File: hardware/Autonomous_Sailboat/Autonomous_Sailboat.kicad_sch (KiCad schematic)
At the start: 16 parts, among them Q1 Q_NMOS, U1 STM32H755ZITx

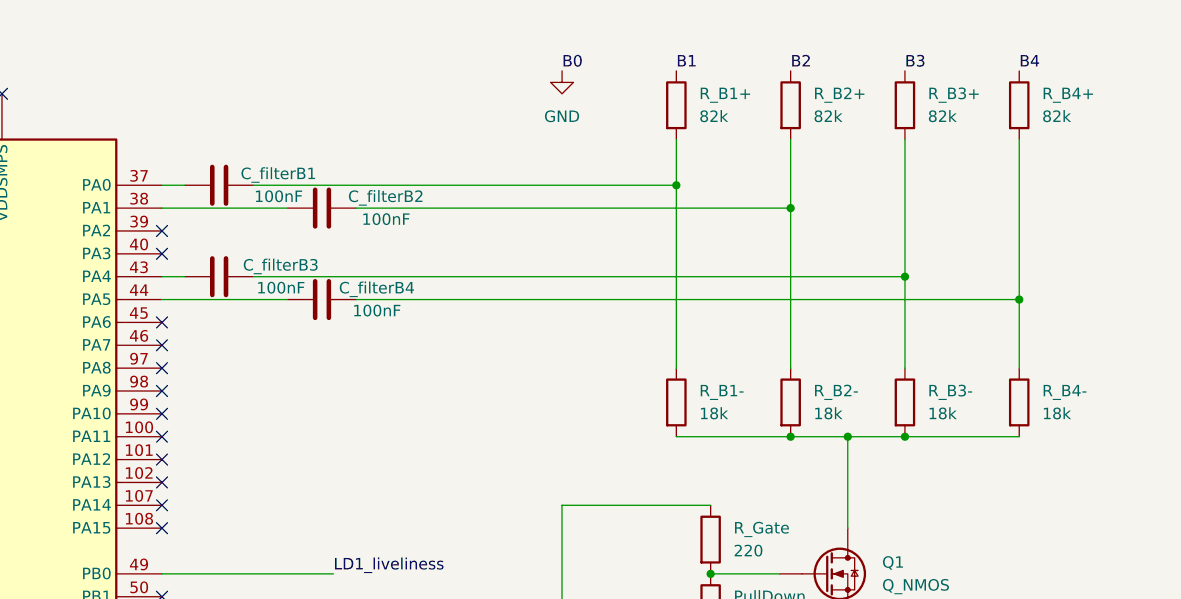
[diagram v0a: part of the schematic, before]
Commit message: naive battery monitor
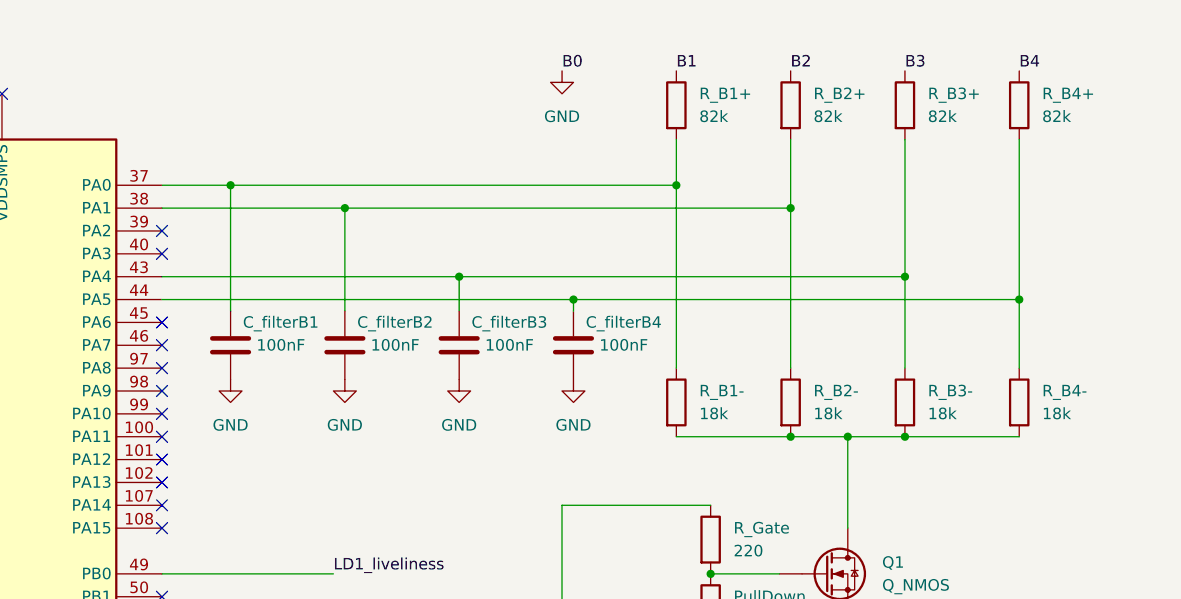
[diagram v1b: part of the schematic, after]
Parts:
- removed C_filterB1: 100nF, symbol Device:C
- added C_filterB2: 100nF, symbol Device:C
- renumbered C_filterB2 to C_filterB1
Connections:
- net GND: now also C_filterB1.1, C_filterB3.1, C_filterB4.1, C_filterB2.1
- net at C_filterB3.2, R_B3+.2, R_B3-.1: now also U1.43 (PA4)
- net at R_B1+.2, R_B1-.1: now also C_filterB1.2, U1.37 (PA0)
- net at C_filterB4.2, R_B4+.2, R_B4-.1: now also U1.44 (PA5)
- net at U1.38 (PA1): now also R_B2+.2, R_B2-.1, C_filterB2.2; no longer C_filterB1.1
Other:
- moved on the sheet: C_filterB1
